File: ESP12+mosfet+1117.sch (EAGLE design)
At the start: 36 parts, among them IC1 LM1117T-3.3-V, Q1 IRLZ34N, Q2 IRLZ34N, Q3 IRLZ34N, Q4 IRLZ34N

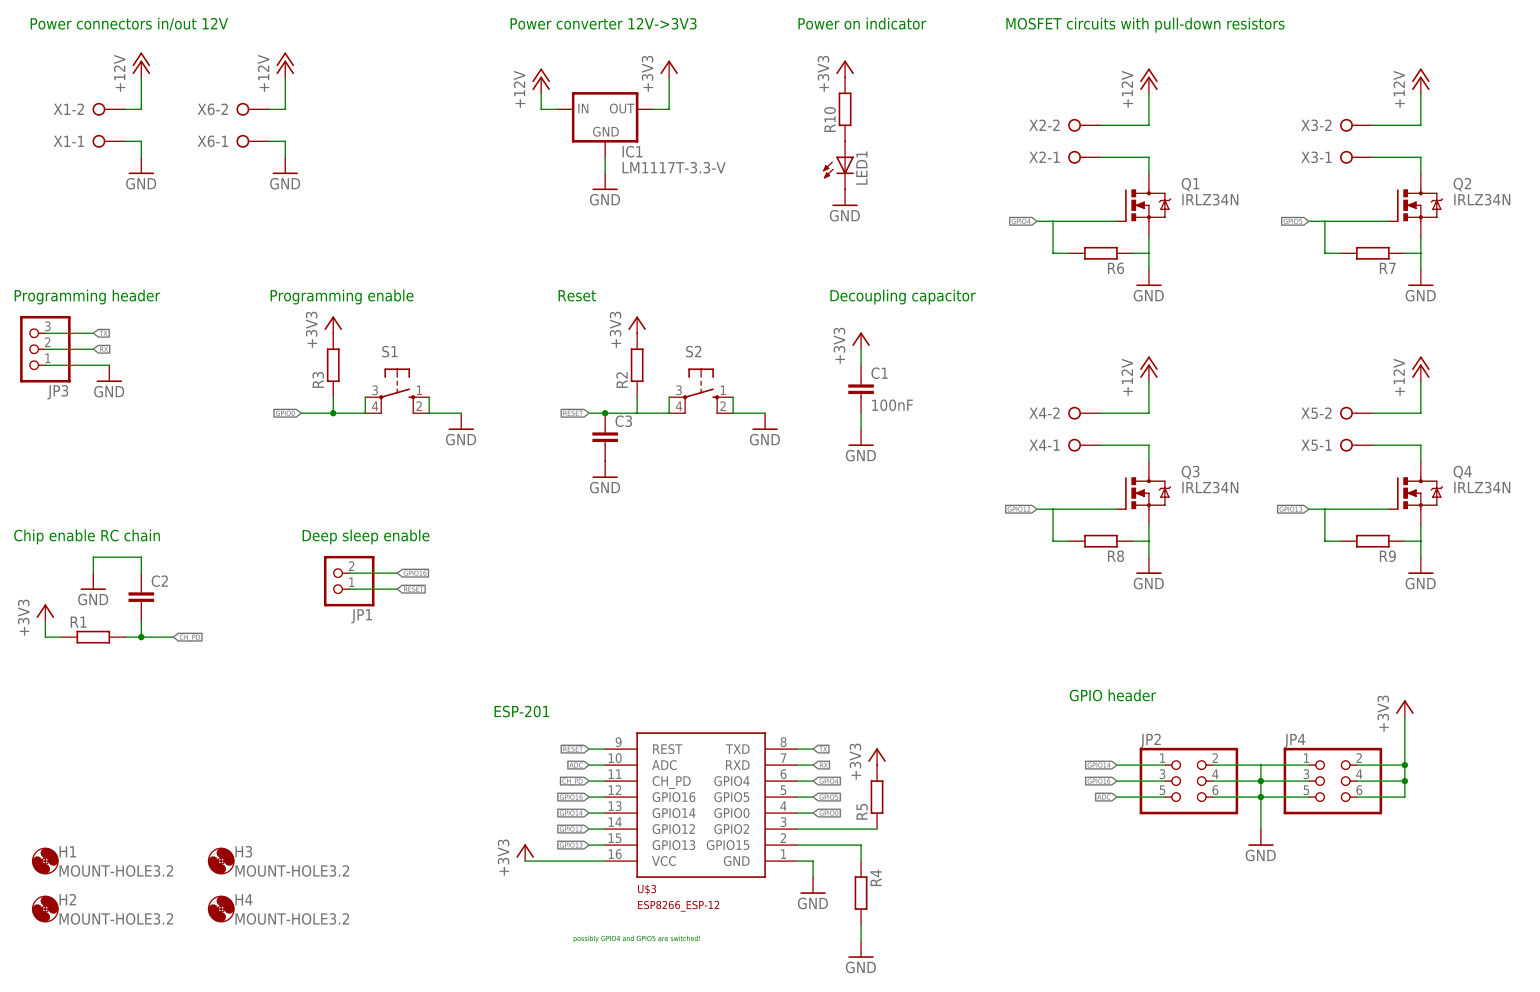
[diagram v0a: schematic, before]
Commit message: New version
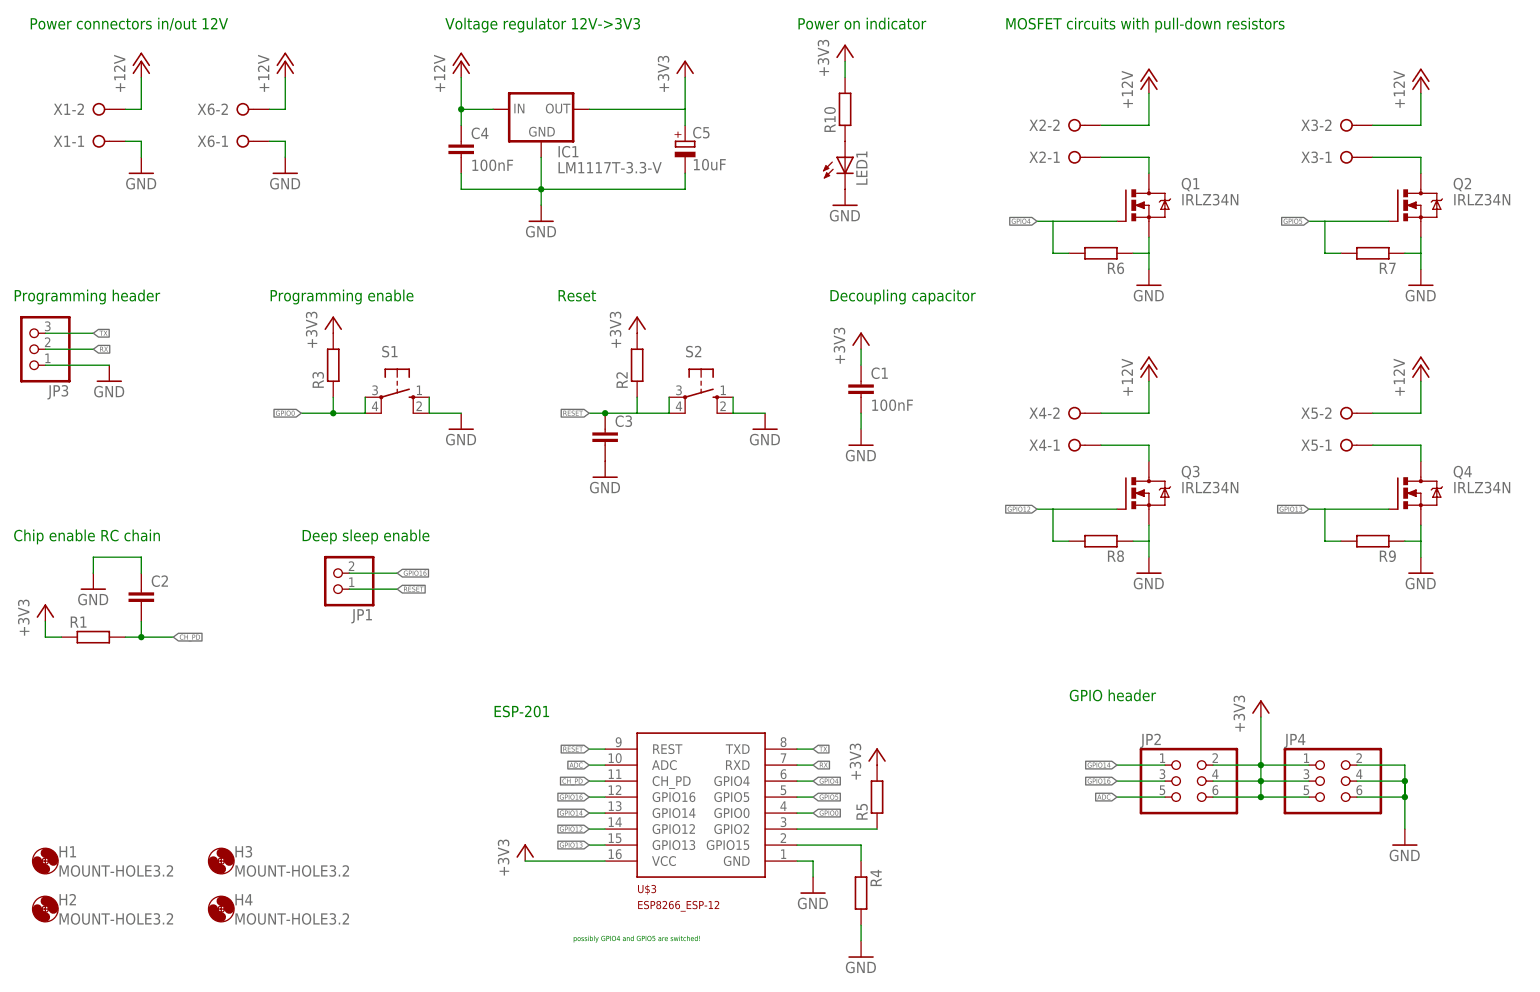
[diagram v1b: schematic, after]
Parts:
- added C4: 100nF, rcl:C-EUC0805
- added C5: 10uF, resistor:CPOL-EUE2-4
- LED1: device led:LED5MM -> led:LED3MM
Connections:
- net +12V: now also C4.1
- net +3V3: now also C5.+, JP2.2, JP2.4, JP2.6, JP4.1, JP4.3, JP4.5; no longer JP4.2, JP4.4, JP4.6
- net GND: now also C4.2, C5.-, JP4.2, JP4.4, JP4.6; no longer JP2.2, JP2.4, JP2.6, JP4.1, JP4.3, JP4.5
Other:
- note added: "Voltage regulator 12V->3V3"
- note removed: "Power converter 12V->3V3"
- moved on the sheet: IC1
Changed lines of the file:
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@@
 <part name="JP2" library="pinhead" deviceset="PINHD-2X3" device=""/>
 <part name="JP4" library="pinhead" deviceset="PINHD-2X3" device=""/>
-<part name="GND17" library="supply1" deviceset="GND" device=""/>
 <part name="+3V4" library="supply1" deviceset="+3V3" device=""/>
 <part name="JP3" library="pinhead" deviceset="PINHD-1X3" device=""/>
@@
 <part name="+3V5" library="supply1" deviceset="+3V3" device=""/>
 <part name="GND18" library="supply1" deviceset="GND" device=""/>
-<part name="LED1" library="led" deviceset="LED" device="5MM"/>
+<part name="LED1" library="led" deviceset="LED" device="3MM"/>
 <part name="+3V2" library="supply1" deviceset="+3V3" device=""/>
 <part name="R10" library="resistor" deviceset="R-EU_" device="0207/10"/>
 <part name="GND3" library="supply1" deviceset="GND" device=""/>
+<part name="C4" library="rcl" deviceset="C-EU" device="C0805" value="100nF"/>
+<part name="C5" library="resistor" deviceset="CPOL-EU" device="E2-4" value="10uF"/>
+<part name="GND4" library="supply1" deviceset="GND" device=""/>
 </parts>
 <sheets>
@@
 <plain>
 <text x="15.24" y="160.02" size="1.778" layer="91">Power connectors in/out 12V</text>
-<text x="91.44" y="160.02" size="1.778" layer="91">Power converter 12V-&gt;3V3</text>
+<text x="81.28" y="160.02" size="1.778" layer="91">Voltage regulator 12V-&gt;3V3</text>
 <text x="142.24" y="116.84" size="1.778" layer="91">Decoupling capacitor</text>
 <text x="12.7" y="116.84" size="1.778" layer="91">Programming header</text>
@@
 <instance part="JP2" gate="A" x="198.12" y="40.64"/>
 <instance part="JP4" gate="A" x="220.98" y="40.64"/>
-<instance part="GND17" gate="1" x="210.82" y="30.48"/>
-<instance part="+3V4" gate="G$1" x="233.68" y="53.34"/>
+<instance part="+3V4" gate="G$1" x="210.82" y="53.34"/>
 <instance part="JP3" gate="A" x="15.24" y="109.22" rot="R180"/>
 <instance part="GND10" gate="1" x="27.94" y="104.14"/>
@@
 <instance part="X6" gate="-1" x="48.26" y="142.24"/>
 <instance part="X6" gate="-2" x="48.26" y="147.32"/>
-<instance part="IC1" gate="G$1" x="106.68" y="147.32"/>
-<instance part="P+8" gate="1" x="96.52" y="152.4"/>
-<instance part="+3V5" gate="G$1" x="116.84" y="154.94"/>
-<instance part="GND18" gate="1" x="106.68" y="134.62"/>
+<instance part="IC1" gate="G$1" x="96.52" y="147.32"/>
+<instance part="P+8" gate="1" x="83.82" y="154.94"/>
+<instance part="+3V5" gate="G$1" x="119.38" y="154.94"/>
+<instance part="GND18" gate="1" x="96.52" y="129.54"/>
 <instance part="LED1" gate="G$1" x="144.78" y="139.7"/>
-<instance part="+3V2" gate="G$1" x="144.78" y="154.94"/>
+<instance part="+3V2" gate="G$1" x="144.78" y="157.48"/>
 <instance part="R10" gate="G$1" x="144.78" y="147.32" rot="R90"/>
 <instance part="GND3" gate="1" x="144.78" y="132.08"/>
+<instance part="C4" gate="G$1" x="83.82" y="142.24"/>
+<instance part="C5" gate="G$1" x="119.38" y="142.24"/>
+<instance part="GND4" gate="1" x="233.68" y="30.48"/>
 </instances>
 <busses>
@@
 </segment>
 <segment>
-<pinref part="JP4" gate="A" pin="1"/>
-<wire x1="218.44" y1="43.18" x2="210.82" y2="43.18" width="0.1524" layer="91"/>
-<wire x1="210.82" y1="43.18" x2="210.82" y2="40.64" width="0.1524" layer="91"/>
-<pinref part="JP2" gate="A" pin="4"/>
-<wire x1="210.82" y1="38.1" x2="210.82" y2="33.02" width="0.1524" layer="91"/>
-<wire x1="203.2" y1="40.64" x2="210.82" y2="40.64" width="0.1524" layer="91"/>
-<pinref part="JP4" gate="A" pin="3"/>
-<wire x1="218.44" y1="40.64" x2="210.82" y2="40.64" width="0.1524" layer="91"/>
-<wire x1="210.82" y1="40.64" x2="210.82" y2="38.1" width="0.1524" layer="91"/>
-<pinref part="JP2" gate="A" pin="6"/>
-<wire x1="203.2" y1="38.1" x2="210.82" y2="38.1" width="0.1524" layer="91"/>
-<pinref part="JP4" gate="A" pin="5"/>
-<wire x1="210.82" y1="38.1" x2="218.44" y2="38.1" width="0.1524" layer="91"/>
-<junction x="210.82" y="40.64"/>
-<junction x="210.82" y="38.1"/>
-<pinref part="GND17" gate="1" pin="GND"/>
-<pinref part="JP2" gate="A" pin="2"/>
-<wire x1="203.2" y1="43.18" x2="210.82" y2="43.18" width="0.1524" layer="91"/>
-</segment>
-<segment>
 <pinref part="JP3" gate="A" pin="1"/>
 <wire x1="17.78" y1="106.68" x2="27.94" y2="106.68" width="0.1524" layer="91"/>
@@
 <pinref part="IC1" gate="G$1" pin="GND"/>
 <pinref part="GND18" gate="1" pin="GND"/>
-<wire x1="106.68" y1="137.16" x2="106.68" y2="139.7" width="0.1524" layer="91"/>
+<wire x1="96.52" y1="132.08" x2="96.52" y2="134.62" width="0.1524" layer="91"/>
+<pinref part="C4" gate="G$1" pin="2"/>
+<wire x1="96.52" y1="134.62" x2="96.52" y2="139.7" width="0.1524" layer="91"/>
+<wire x1="83.82" y1="137.16" x2="83.82" y2="134.62" width="0.1524" layer="91"/>
+<wire x1="83.82" y1="134.62" x2="96.52" y2="134.62" width="0.1524" layer="91"/>
+<junction x="96.52" y="134.62"/>
+<pinref part="C5" gate="G$1" pin="-"/>
+<wire x1="96.52" y1="134.62" x2="119.38" y2="134.62" width="0.1524" layer="91"/>
+<wire x1="119.38" y1="134.62" x2="119.38" y2="137.16" width="0.1524" layer="91"/>
 </segment>
 <segment>
 <pinref part="GND3" gate="1" pin="GND"/>
 <pinref part="LED1" gate="G$1" pin="C"/>
+</segment>
+<segment>
+<pinref part="JP4" gate="A" pin="2"/>
+<wire x1="226.06" y1="43.18" x2="233.68" y2="43.18" width="0.1524" layer="91"/>
+<pinref part="GND4" gate="1" pin="GND"/>
+<wire x1="233.68" y1="43.18" x2="233.68" y2="40.64" width="0.1524" layer="91"/>
+<pinref part="JP4" gate="A" pin="6"/>
+<wire x1="233.68" y1="40.64" x2="233.68" y2="38.1" width="0.1524" layer="91"/>
+<wire x1="233.68" y1="38.1" x2="233.68" y2="33.02" width="0.1524" layer="91"/>
+<wire x1="226.06" y1="38.1" x2="233.68" y2="38.1" width="0.1524" layer="91"/>
+<wire x1="233.68" y1="38.1" x2="233.68" y2="40.64" width="0.1524" layer="91"/>
+<pinref part="JP4" gate="A" pin="4"/>
+<wire x1="226.06" y1="40.64" x2="233.68" y2="40.64" width="0.1524" layer="91"/>
+<junction x="233.68" y="40.64"/>
+<junction x="233.68" y="38.1"/>
 </segment>
 </net>
@@
 <pinref part="IC1" gate="G$1" pin="IN"/>
 <pinref part="P+8" gate="1" pin="+12V"/>
-<wire x1="99.06" y1="147.32" x2="96.52" y2="147.32" width="0.1524" layer="91"/>
-<wire x1="96.52" y1="147.32" x2="96.52" y2="149.86" width="0.1524" layer="91"/>
+<wire x1="83.82" y1="147.32" x2="83.82" y2="152.4" width="0.1524" layer="91"/>
+<pinref part="C4" gate="G$1" pin="1"/>
+<wire x1="83.82" y1="144.78" x2="83.82" y2="147.32" width="0.1524" layer="91"/>
+<wire x1="83.82" y1="147.32" x2="88.9" y2="147.32" width="0.1524" layer="91"/>
+<junction x="83.82" y="147.32"/>
 </segment>
 </net>
@@
 </segment>
 <segment>
-<pinref part="JP4" gate="A" pin="6"/>
-<wire x1="226.06" y1="38.1" x2="233.68" y2="38.1" width="0.1524" layer="91"/>
-<wire x1="233.68" y1="38.1" x2="233.68" y2="40.64" width="0.1524" layer="91"/>
-<pinref part="JP4" gate="A" pin="4"/>
-<wire x1="233.68" y1="40.64" x2="233.68" y2="43.18" width="0.1524" layer="91"/>
-<wire x1="233.68" y1="43.18" x2="233.68" y2="50.8" width="0.1524" layer="91"/>
-<wire x1="226.06" y1="40.64" x2="233.68" y2="40.64" width="0.1524" layer="91"/>
-<pinref part="JP4" gate="A" pin="2"/>
-<wire x1="226.06" y1="43.18" x2="233.68" y2="43.18" width="0.1524" layer="91"/>
-<pinref part="+3V4" gate="G$1" pin="+3V3"/>
-<junction x="233.68" y="40.64"/>
-<junction x="233.68" y="43.18"/>
-</segment>
-<segment>
 <pinref part="IC1" gate="G$1" pin="OUT"/>
 <pinref part="+3V5" gate="G$1" pin="+3V3"/>
-<wire x1="114.3" y1="147.32" x2="116.84" y2="147.32" width="0.1524" layer="91"/>
-<wire x1="116.84" y1="147.32" x2="116.84" y2="152.4" width="0.1524" layer="91"/>
+<wire x1="104.14" y1="147.32" x2="119.38" y2="147.32" width="0.1524" layer="91"/>
+<wire x1="119.38" y1="147.32" x2="119.38" y2="152.4" width="0.1524" layer="91"/>
+<pinref part="C5" gate="G$1" pin="+"/>
+<wire x1="119.38" y1="144.78" x2="119.38" y2="147.32" width="0.1524" layer="91"/>
 </segment>
 <segment>
 <pinref part="R10" gate="G$1" pin="2"/>
 <pinref part="+3V2" gate="G$1" pin="+3V3"/>
+<wire x1="144.78" y1="154.94" x2="144.78" y2="152.4" width="0.1524" layer="91"/>
+</segment>
+<segment>
+<pinref part="JP4" gate="A" pin="1"/>
+<wire x1="218.44" y1="43.18" x2="210.82" y2="43.18" width="0.1524" layer="91"/>
+<wire x1="210.82" y1="43.18" x2="210.82" y2="40.64" width="0.1524" layer="91"/>
+<pinref part="JP2" gate="A" pin="4"/>
+<wire x1="203.2" y1="40.64" x2="210.82" y2="40.64" width="0.1524" layer="91"/>
+<pinref part="JP4" gate="A" pin="3"/>
+<wire x1="218.44" y1="40.64" x2="210.82" y2="40.64" width="0.1524" layer="91"/>
+<wire x1="210.82" y1="40.64" x2="210.82" y2="38.1" width="0.1524" layer="91"/>
+<junction x="210.82" y="40.64"/>
+<pinref part="JP2" gate="A" pin="2"/>
+<wire x1="203.2" y1="43.18" x2="210.82" y2="43.18" width="0.1524" layer="91"/>
+<pinref part="+3V4" gate="G$1" pin="+3V3"/>
+<wire x1="210.82" y1="43.18" x2="210.82" y2="50.8" width="0.1524" layer="91"/>
+<junction x="210.82" y="43.18"/>
+<pinref part="JP4" gate="A" pin="5"/>
+<pinref part="JP2" gate="A" pin="6"/>
+<wire x1="203.2" y1="38.1" x2="210.82" y2="38.1" width="0.1524" layer="91"/>
+<junction x="210.82" y="38.1"/>
+<wire x1="210.82" y1="38.1" x2="218.44" y2="38.1" width="0.1524" layer="91"/>
 </segment>
 </net>
